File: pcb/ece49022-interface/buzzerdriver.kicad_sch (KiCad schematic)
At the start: 4 parts, among them Q1 C1815

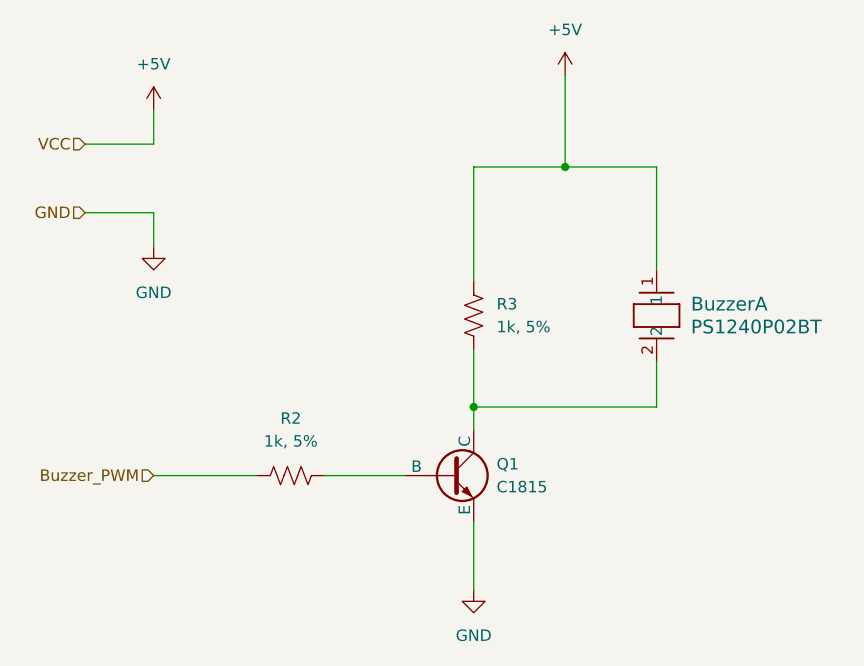
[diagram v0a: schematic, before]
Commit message: Interface
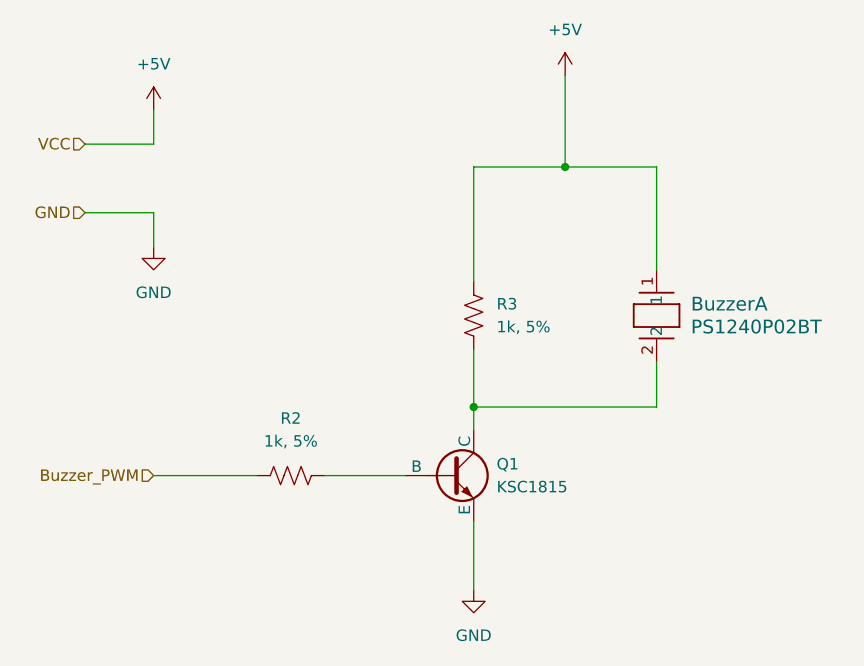
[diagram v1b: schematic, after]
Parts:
- Q1: value C1815 -> KSC1815
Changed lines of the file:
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@@
 			)
 		)
-		(property "Value" "C1815"
+		(property "Value" "KSC1815"
 			(at 130.81 110.4899 0)
 			(effects
@@
 			)
 		)
-		(property "Description" "5399-C1815CT-ND"
+		(property "Description" "KSC1815YTA"
 			(at 125.73 109.22 0)
 			(effects

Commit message: footprint update
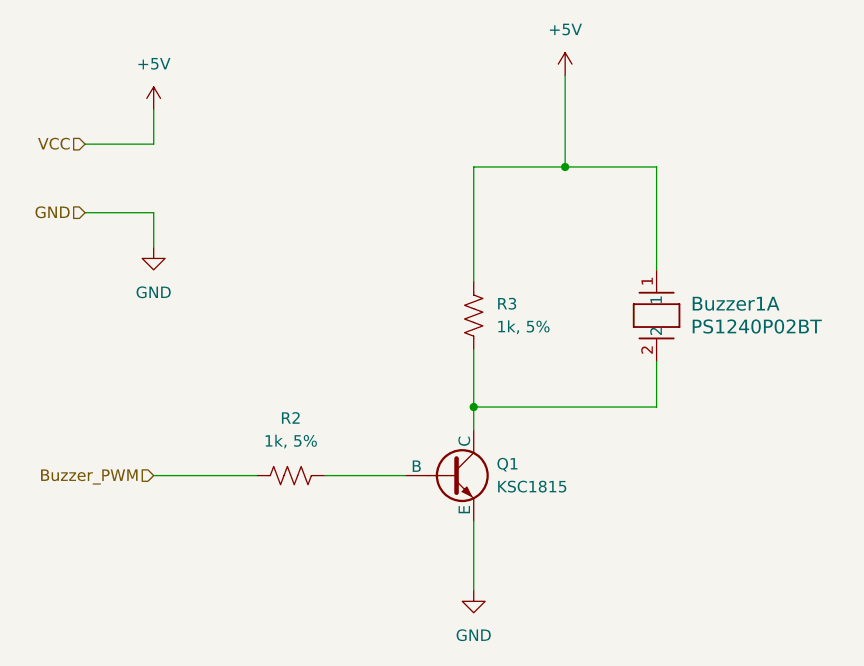
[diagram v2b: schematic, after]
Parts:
- R2, R3: footprint (none) -> Resistor_SMD:R_0402_1005Metric
- renumbered Buzzer to Buzzer1
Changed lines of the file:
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@@
 		(dnp no)
 		(fields_autoplaced yes)
-		(property "Reference" "Buzzer"
+		(property "Reference" "Buzzer1"
 			(at 152.4 90.1699 90)
 			(effects
@@
 			(project "ece49022-interface"
 				(path "/ad062fbe-cbe6-4ffd-876d-97a59a1c7176/6d9997a2-880e-441e-bac1-2563afa1369d"
-					(reference "Buzzer")
+					(reference "Buzzer1")
 					(unit 1)
 				)
@@
 			)
 		)
-		(property "Footprint" ""
+		(property "Footprint" "Resistor_SMD:R_0402_1005Metric"
 			(at 127.254 91.186 90)
 			(effects
@@
 			)
 		)
-		(property "Footprint" ""
+		(property "Footprint" "Resistor_SMD:R_0402_1005Metric"
 			(at 108.204 108.204 90)
 			(effects
